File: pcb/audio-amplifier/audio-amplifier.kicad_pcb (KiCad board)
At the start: 4 copper layers, 100 x 81 mm, 71 parts, among them J1 PJ-320D, J2 WJ500V-5.08-2P, J3 WJ500V-5.08-2P, J4 WJ500V-5.08-2P, Q1 IRFR4615TRLPBF, Q2 IRFR4615TRLPBF, Q3 IRFR4615TRLPBF, Q4 IRFR4615TRLPBF, U1 LMC555M, U10 DGD05473, U2 COS2353SR, U3 COS2353SR, U4 COS2353SR, U5 TLV3201, U6 TLV3201, U7 74LVC1G04SE, U8 DGD05473, U9 74LVC1G04SE

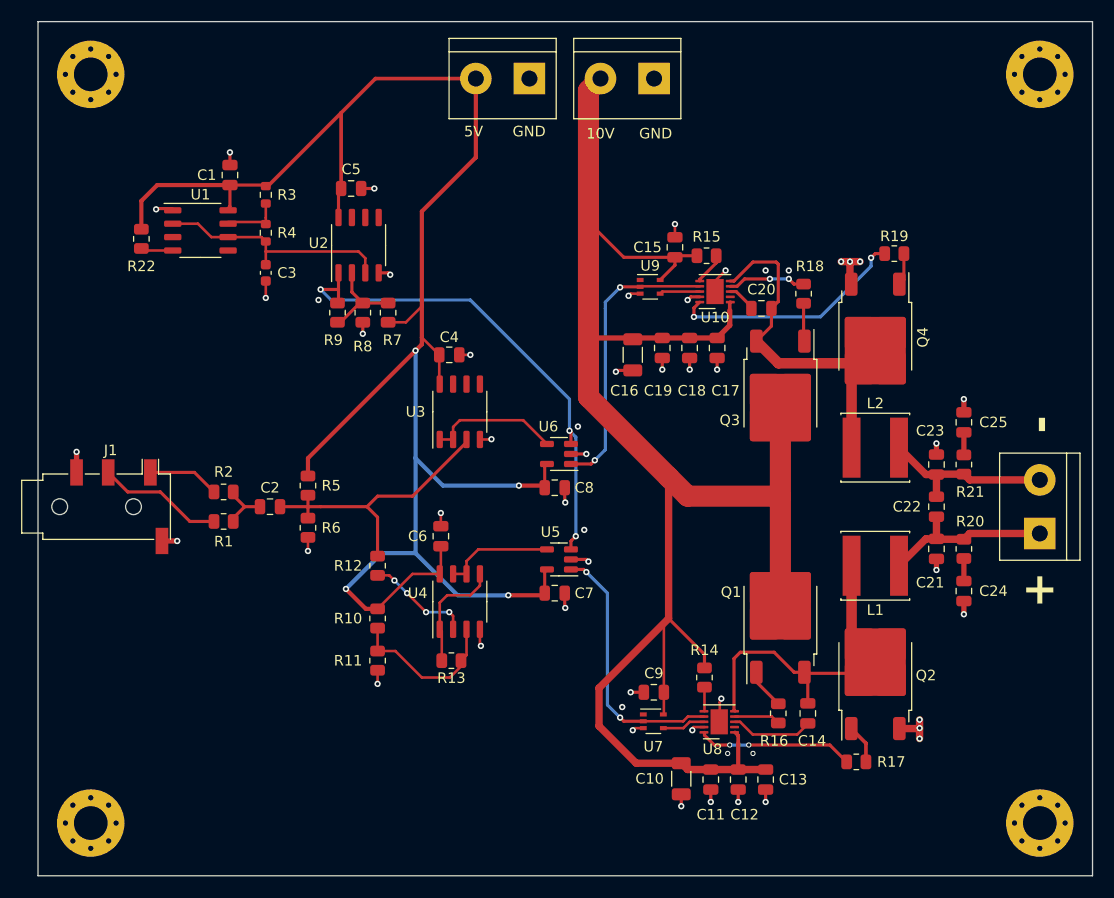
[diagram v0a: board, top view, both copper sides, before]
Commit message: Add updated PCB
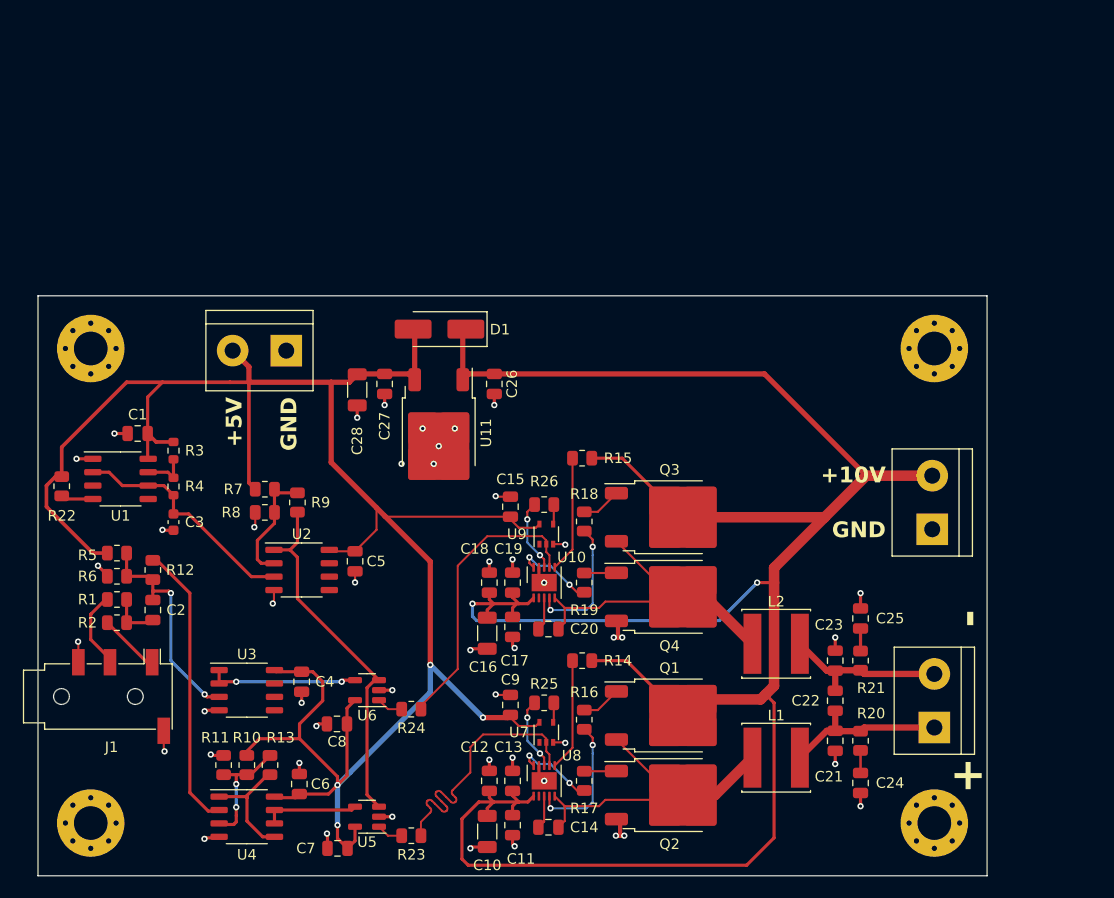
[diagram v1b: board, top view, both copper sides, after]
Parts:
- added C26: 330nF, Capacitor_SMD:C_0805_2012Metric, F.Cu at (143.3, 72.4)
- added C27: 100nF, Capacitor_SMD:C_0805_2012Metric, F.Cu at (132.9, 72.4)
- added C28: 4.7uF, Capacitor_SMD:C_1206_3216Metric, F.Cu at (130.3, 72.9)
- added D1: SS54, Diode_SMD:D_SMA_Handsoldering, F.Cu at (138.1, 67.2)
- added R23: 50R, Resistor_SMD:R_0805_2012Metric, F.Cu at (135.4, 115.2)
- added R24: 50R, Resistor_SMD:R_0805_2012Metric, F.Cu at (135.4, 103.2)
- added R25: 50R, Resistor_SMD:R_0805_2012Metric, F.Cu at (148.0, 102.6)
- added R26: 50R, Resistor_SMD:R_0805_2012Metric, F.Cu at (148.0, 83.8)
- added U11: LDO_L78M05CDT_SOT89, Package_TO_SOT_SMD:TO-252-2, F.Cu at (138.0, 77.0)
- R7, R8: value R -> 226K
- moved J3 50.2 mm to (184.8, 86.1), turned to 90 degrees
- moved R19 42.9 mm to (151.8, 91.2), turned to 90 degrees
- moved C20 36.5 mm to (148.4, 95.6)
- moved C5 35.4 mm to (130.1, 89.2), turned to -90 degrees
- moved J2 34.6 mm to (123.5, 69.2)
- moved C4 34.0 mm to (125.0, 100.6), turned to -90 degrees
- moved U3 33.2 mm to (119.8, 101.4), turned to 0 degrees
- moved C17 32.8 mm to (145.0, 95.4)
- moved U10 32.0 mm to (148.0, 91.2), turned to 90 degrees
- moved C7 31.8 mm to (128.4, 116.4), turned to 180 degrees
- moved Q4 31.4 mm to (159.9, 92.5), turned to 0 degrees
- moved U2 31.3 mm to (125.0, 90.0), turned to 0 degrees
- moved C8 30.5 mm to (128.3, 104.6), turned to 180 degrees
- moved U5 30.4 mm to (131.2, 113.4)
- moved R18 30.0 mm to (151.8, 85.4), turned to 90 degrees
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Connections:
- C15 pad 1: +10V -> +5V
- C9 pad 1: +10V -> +5V
- U5 pad 1: /Half Bridge Driver Left/PWM -> Net-(R23-Pad1)
- U6 pad 1: /Half Bridge Driver Right/PWM -> Net-(R24-Pad1)
- U7 pad 1: (no net) -> unconnected-(U7-NC-Pad1)
- U7 pad 4: Net-(U8-LIN) -> Net-(R25-Pad1)
- U7 pad 5: +10V -> +5V
- U9 pad 1: (no net) -> unconnected-(U9-NC-Pad1)
- U9 pad 4: Net-(U10-LIN) -> Net-(R26-Pad1)
- U9 pad 5: +10V -> +5V
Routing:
- net +10V: track 165.1 -> 220.2 mm, vias 0 -> 2
- net +5V: track 177.9 -> 209.2 mm
- net Net-(U4A--): track 10.0 -> 27.2 mm, vias 4 -> 0
- net Net-(U10-LO): track 22.7 -> 7.69 mm
- net /TRIANGLE: track 48.5 -> 34.4 mm, vias 3 -> 0
- net /Half Bridge Driver Left/EN: track 2.29 -> 10.6 mm
- net Net-(U8-HO): track 4.35 -> 12.7 mm, vias 0 -> 2
- net /Half Bridge Driver Right/EN: track 3.05 -> 11.0 mm
- net Net-(U8-LO): track 14.8 -> 7.69 mm
- net Net-(U3A-+): track 27.8 -> 20.9 mm, vias 0 -> 2
- net Net-(U10-HO): track 7.44 -> 12.7 mm
- net Net-(U8-VB): track 7.91 -> 3.18 mm
- net Net-(J1-PadR1): track 12.0 -> 7.46 mm
- net Net-(U4A-+): track 15.3 -> 11.4 mm, vias 0 -> 2
- net Net-(U10-LIN): track 3.83 -> 6.90 mm, vias 0 -> 2
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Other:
- board size 100 x 81 mm -> 90 x 55 mm
- board text added: "+10V"
- board text added: "+5V"
- board text removed: "10V"
- board text removed: "5V"
